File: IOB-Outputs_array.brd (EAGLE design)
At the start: 61 x 81.3 mm, 64 parts, among them Q1X11 MOSFET-N, Q1X12 MOSFET-N, Q1X13 MOSFET-N, Q1X14 MOSFET-N, Q2X11 MOSFET-N, Q2X12 MOSFET-N, Q2X13 MOSFET-N, Q2X14 MOSFET-N, Q3X11 MOSFET-N, Q3X12 MOSFET-N, Q3X13 MOSFET-N, Q3X14 MOSFET-N, Q4X11 MOSFET-N, Q4X12 MOSFET-N, Q4X13 MOSFET-N, Q4X14 MOSFET-N, Q5X11 MOSFET-N, Q5X12 MOSFET-N, Q5X13 MOSFET-N, Q5X14 MOSFET-N, Q6X11 MOSFET-N, Q6X12 MOSFET-N, Q6X13 MOSFET-N, Q6X14 MOSFET-N, Q7X11 MOSFET-N, Q7X12 MOSFET-N, Q7X13 MOSFET-N, Q7X14 MOSFET-N, Q8X11 MOSFET-N, Q8X12 MOSFET-N, Q8X13 MOSFET-N, Q8X14 MOSFET-N

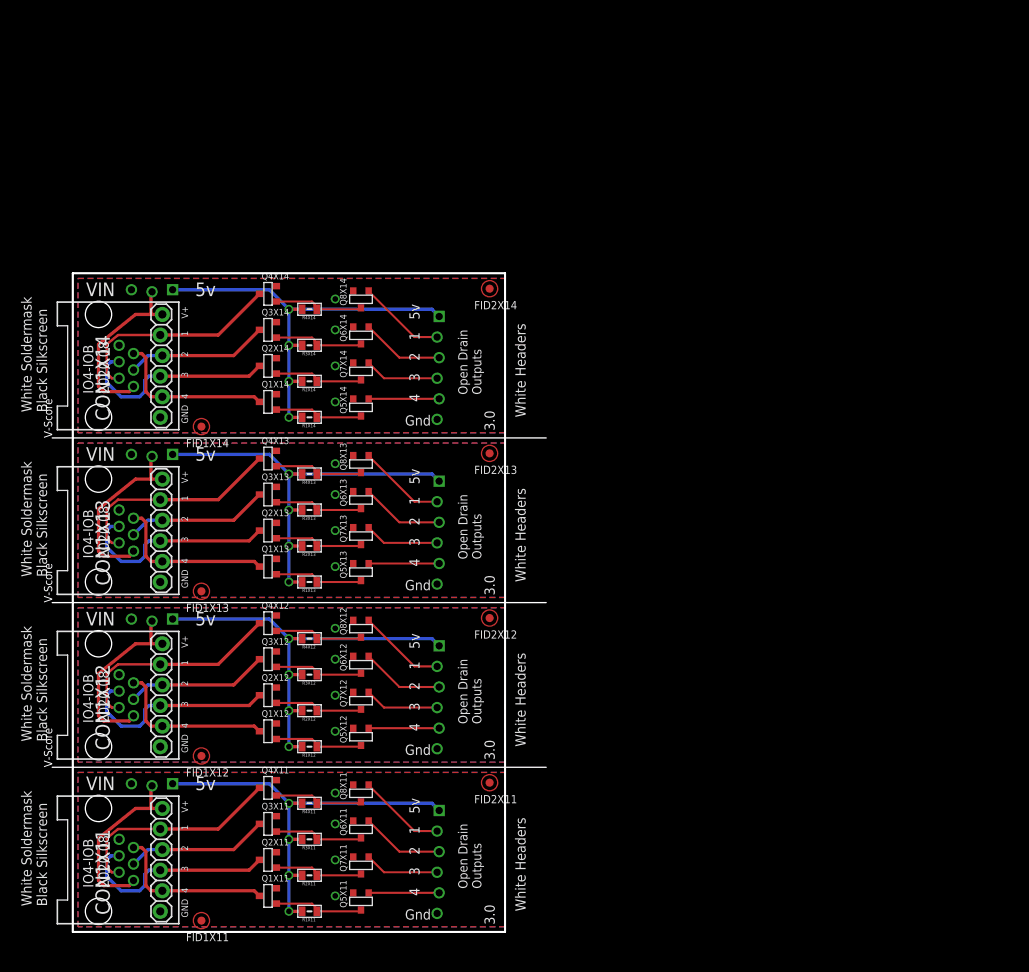
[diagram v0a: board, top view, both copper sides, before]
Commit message: added board template
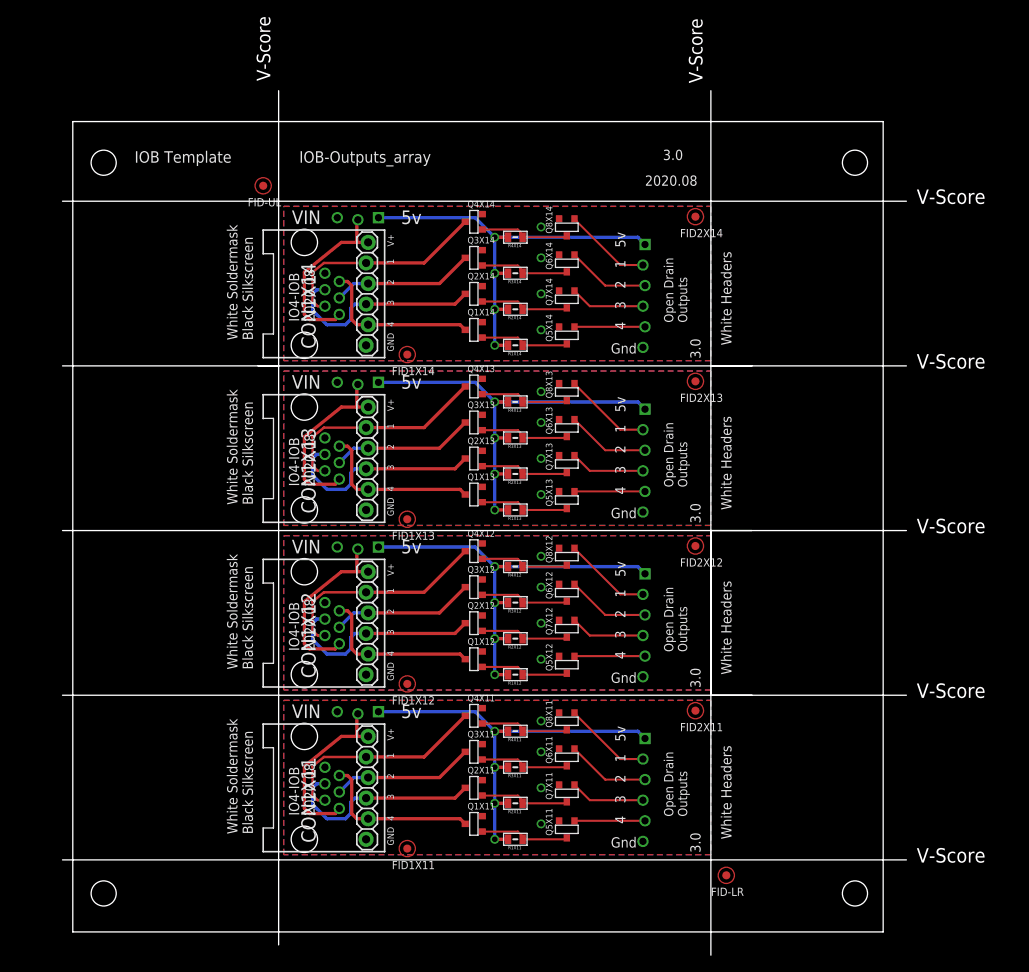
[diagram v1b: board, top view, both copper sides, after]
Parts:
- added FID-LR, FID-UL: FIDUCIAL, SPCoast:FIDUCIAL_1MM
- added R8X1: (no value), SPCoast:BOARD-DINRAIL-3.17IN-H4X-IOB
- moved Q1X11 26.9 mm to (49.5, 13.3)
- moved Q1X12 26.9 mm to (49.5, 33.7)
- moved Q1X13 26.9 mm to (49.5, 54.0)
- moved Q1X14 26.9 mm to (49.5, 74.3)
- moved Q2X11 26.9 mm to (49.5, 17.8)
- moved Q2X12 26.9 mm to (49.5, 38.1)
- moved Q2X13 26.9 mm to (49.5, 58.4)
- moved Q2X14 26.9 mm to (49.5, 78.7)
- moved Q3X11 26.9 mm to (49.5, 22.2)
- moved Q3X12 26.9 mm to (49.5, 42.5)
- moved Q3X13 26.9 mm to (49.5, 62.9)
- moved Q3X14 26.9 mm to (49.5, 83.2)
- moved Q4X11 26.9 mm to (49.5, 26.7)
- moved Q4X12 26.9 mm to (49.5, 47.0)
- moved Q4X13 26.9 mm to (49.5, 67.3)
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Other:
- board size 61 x 81.3 mm -> 104.1 x 106.7 mm
- board text removed: "V-Score"
